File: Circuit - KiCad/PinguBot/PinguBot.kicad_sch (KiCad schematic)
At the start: 28 parts, among them J1 Jack-DC, Q1 2N2219, U1 LM386, U2 DRV8833PW, U3 LM7805_TO220, U4 TSOP45xx, U5 ESP32_DEVKITC

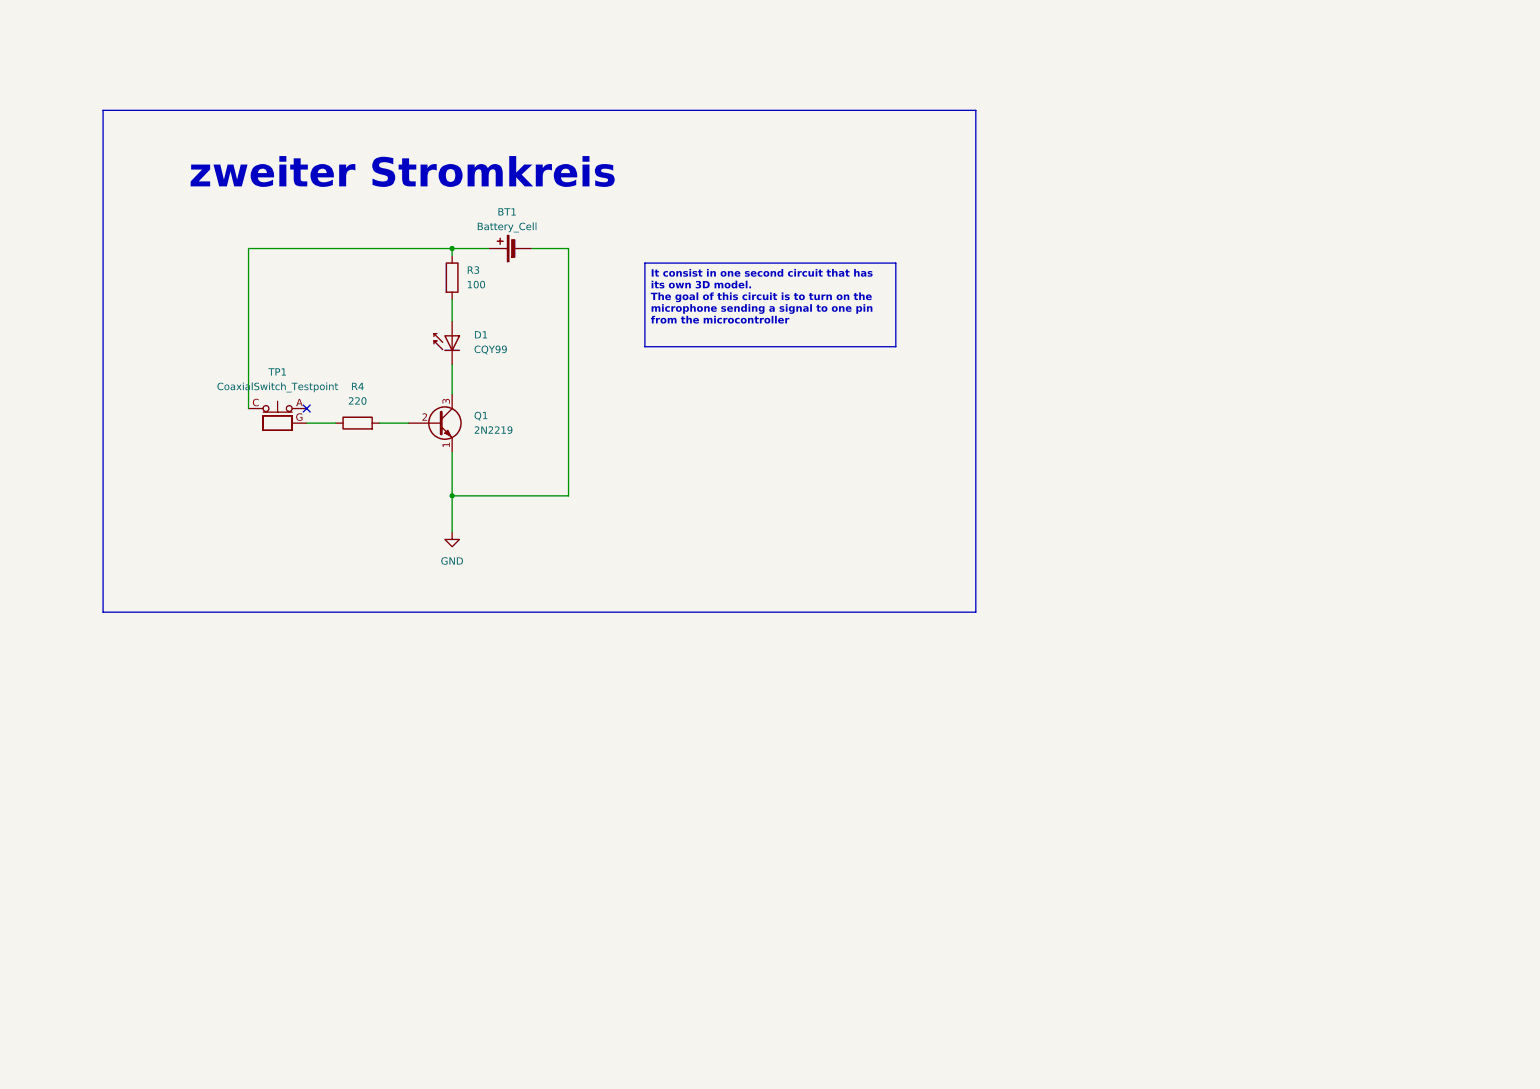
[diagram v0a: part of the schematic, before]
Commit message: Circuit Improvement
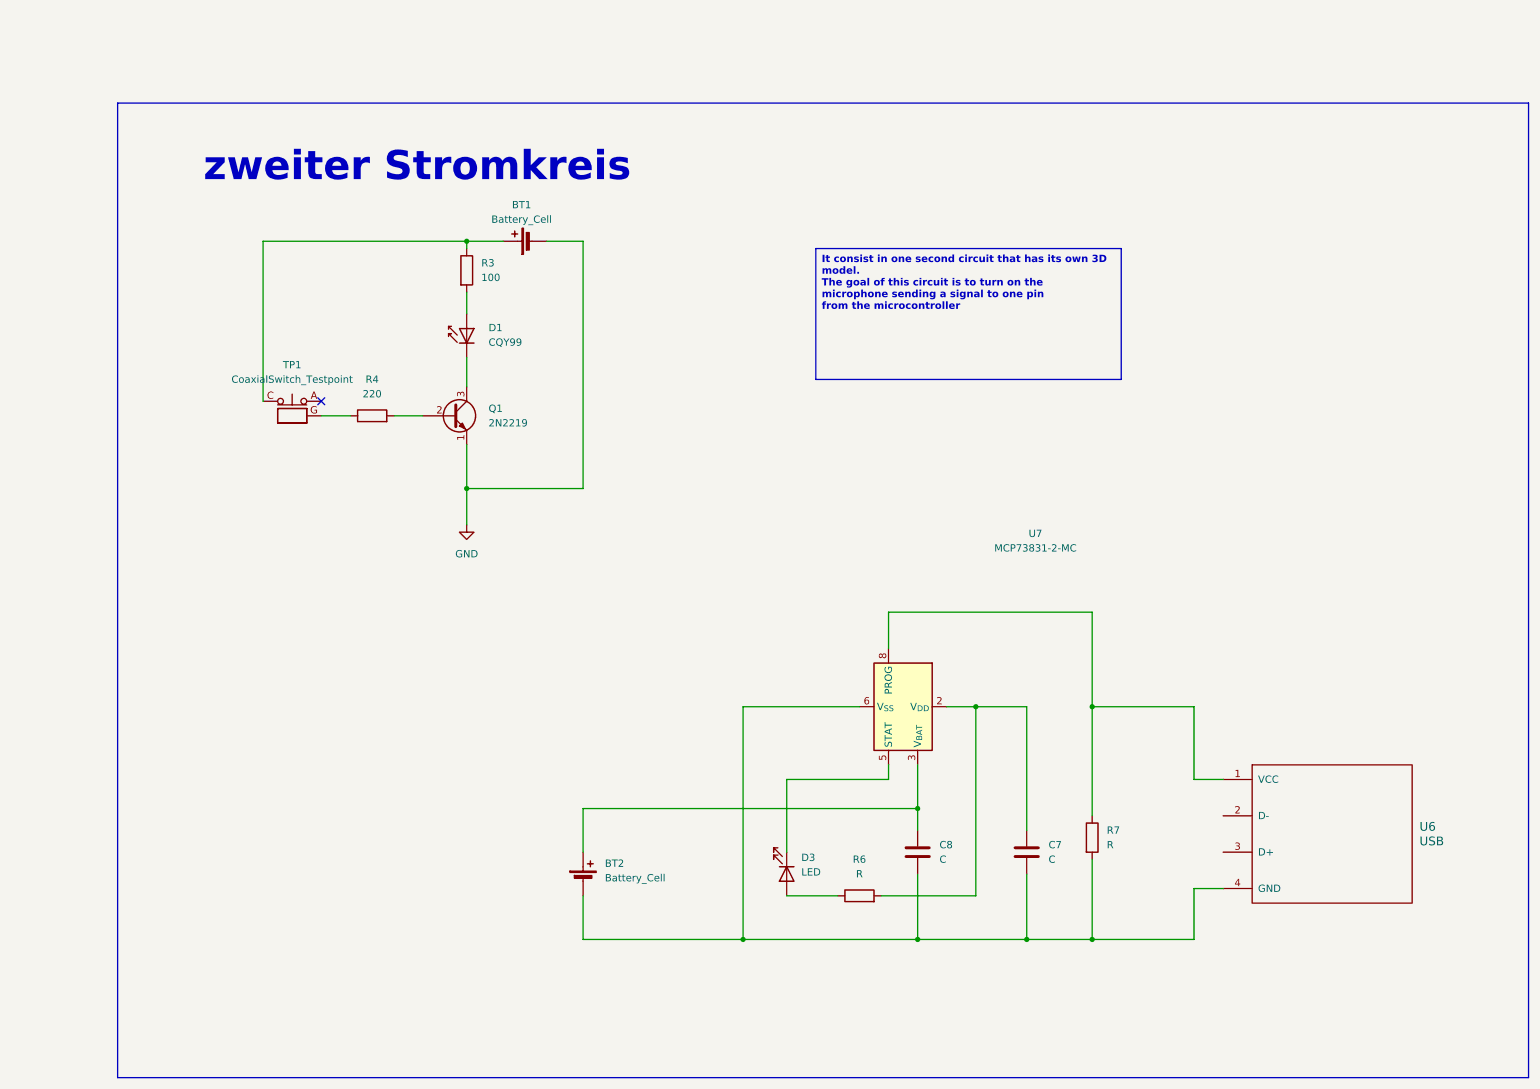
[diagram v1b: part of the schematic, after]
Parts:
- added BT2: Battery_Cell, symbol Device:Battery_Cell
- added C7, C8: C, symbol Device:C
- added D3: LED, symbol Device:LED
- added R6, R7: R, symbol Device:R
- added U6: USB, symbol EESTN5:USB
- added U7: MCP73831-2-MC, Package_DFN_QFN:DFN-8-1EP_3x2mm_P0.5mm_EP1.7x1.4mm, symbol Battery_Management:MCP73831-2-MC
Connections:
- new net: R7.1, U6.1 (VCC), U7.8 (PROG)
- new net: BT2.2 (-), C7.2, C8.2, R7.2, U6.4 (GND), U7.6 (V_{SS})
- new net: D3.2 (A), R6.1
- new net: C7.1, R6.2, U7.1 (V_{DD}), U7.2 (V_{DD})
- new net: D3.1 (K), U7.5 (STAT)
- new net: BT2.1 (+), C8.1, U7.3 (V_{BAT}), U7.4 (V_{BAT})
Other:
- moved on the sheet: BT1, D1, Q1, R3, R4, TP1

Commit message: Circuit Improvement
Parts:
- removed BT1, BT2: Battery_Cell, symbol Device:Battery_Cell
- removed C7, C8: C, symbol Device:C
- removed D1: CQY99, LED_THT:LED_D5.0mm_IRGrey, symbol LED:CQY99
- removed D3: LED, symbol Device:LED
- removed Q1: 2N2219, Package_TO_SOT_THT:TO-39-3, symbol Transistor_BJT:2N2219
- removed R3: 100, symbol Device:R
- removed R4: 220, symbol Device:R
- removed R6, R7: R, symbol Device:R
- removed TP1: CoaxialSwitch_Testpoint, symbol Connector:CoaxialSwitch_Testpoint
- removed U2: DRV8833PW, Package_SO:TSSOP-16_4.4x5mm_P0.65mm, symbol Driver_Motor:DRV8833PW
- removed U6: USB, symbol EESTN5:USB
- removed U7: MCP73831-2-MC, Package_DFN_QFN:DFN-8-1EP_3x2mm_P0.5mm_EP1.7x1.4mm, symbol Battery_Management:MCP73831-2-MC
- added J2, J3: Conn_01x08_Pin, symbol Connector:Conn_01x08_Pin
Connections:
- net 5V: now also ServoMotorOne.3 (Pin_3), ServoMotorTwo.3 (Pin_3), J2.8 (Pin_8)
- net GND: now also Microphone.2 (Pin_2), ServoMotorOne.2 (Pin_2), ServoMotorTwo.2 (Pin_2), J2.1 (Pin_1), J2.6 (Pin_6), J3.1 (Pin_1)
- net MA1: now also J3.6 (Pin_6)
- net MA2: now also J3.7 (Pin_7)
- net MB1: now also J3.4 (Pin_4)
- net MB2: now also J3.3 (Pin_3)
- net STBY: now also J3.5 (Pin_5)
- net MO2: now reaches MotorOne.1 (Pin_1)
- net MO2: now also J2.4 (Pin_4)
- net MO1: now reaches MotorOne.2 (Pin_2)
- net MO1: now also J2.5 (Pin_5)
- net MO4: now reaches MotorTwo.1 (Pin_1)
- net MO4: now also J2.2 (Pin_2)
- net MO3: now reaches MotorTwo.2 (Pin_2)
- net MO3: now also J2.3 (Pin_3)
- net Microphone ADC: now reaches Microphone.1 (Pin_1)
- net Microphone ADC: now also U5.8 (IO33)
- net S_Motor_OUT_1: now reaches U5.11 (IO27)
- net S_Motor_OUT_1: now also ServoMotorTwo.1 (Pin_1)
- net S_Motor_OUT_2: now reaches U5.12 (IO14)
- net S_Motor_OUT_2: now also ServoMotorOne.1 (Pin_1)
- net Speaker DAC: now reaches U5.9 (IO25)
- net Speaker DAC: now also R2.1
- net Microphone RX: no longer names the net of U5.34 (RXD0)
- net Speaker TX: no longer names the net of U5.35 (TXD0)
- net Speaker TX: no longer R2.1
- no-connect marks 2 -> 27
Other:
- note added: "Dual H-Bridge and DC Motors"
- note added: "IR Receiver"
- note removed: "zweiter Stromkreis"
- moved on the sheet: C1, C2, C3, MotorOne, MotorTwo, R1, R2, ServoMotorOne, ServoMotorTwo, Speaker, U1, U4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
